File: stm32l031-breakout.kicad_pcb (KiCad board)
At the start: 2 copper layers, 12 parts, among them J1 Conn_01x16, J2 Conn_01x16, U1 STM32L031K6Tx

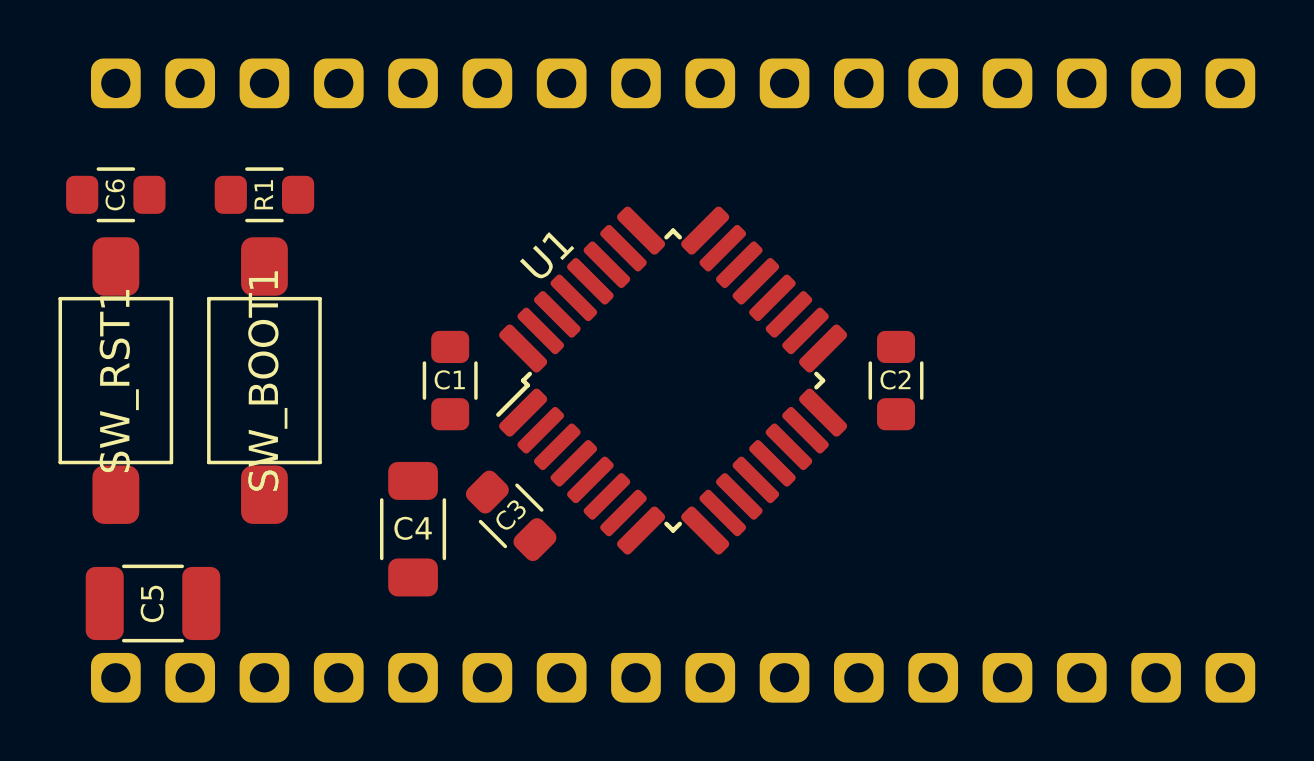
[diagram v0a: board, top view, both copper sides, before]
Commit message: Placement candidate
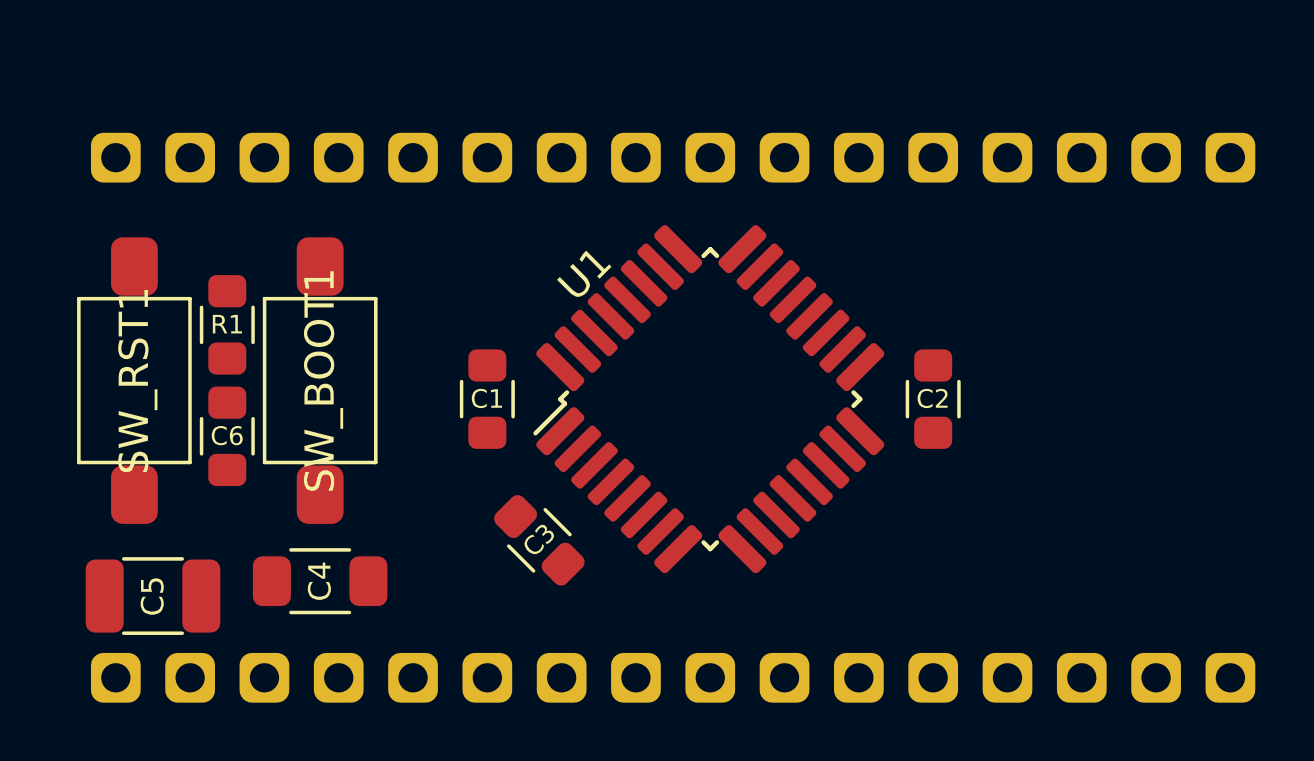
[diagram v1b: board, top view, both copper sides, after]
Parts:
- moved C6 9.09 mm to (143.5, 113.7), turned to 90 degrees
- moved R1 4.62 mm to (143.5, 109.9), turned to 270 degrees
- moved C4 3.64 mm to (146.7, 118.6), turned to 180 degrees
- moved J2 2.54 mm to (139.7, 104.1)
- moved SW_BOOT1 1.91 mm to (146.7, 111.8)
- moved C1 1.42 mm to (152.4, 112.4)
- moved U1 1.42 mm to (160.0, 112.4)
- moved C2 1.42 mm to (167.6, 112.4)
- moved C3 1.28 mm to (154.2, 117.2)
- moved SW_RST1 0.64 mm to (140.3, 111.8), turned to 270 degrees
- moved C5 0.25 mm to (141.0, 119.1)
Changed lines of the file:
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@@
   )
   (module local_footprints:0805_HS (layer F.Cu)
-    (at 151.13 111.76 90)
+    (at 152.4 112.395 90)
     (descr "Resistor SMD 0805, reflow soldering, Vishay (see dcrcw.pdf)")
     (tags "resistor 0805")
@@
   )
   (module local_footprints:0805_HS (layer F.Cu)
-    (at 166.37 111.76 270)
+    (at 167.64 112.395 270)
     (descr "Resistor SMD 0805, reflow soldering, Vishay (see dcrcw.pdf)")
     (tags "resistor 0805")
@@
   )
   (module local_footprints:0805_HS (layer F.Cu)
-    (at 153.213173 116.383173 135)
+    (at 154.178 117.221 135)
     (descr "Resistor SMD 0805, reflow soldering, Vishay (see dcrcw.pdf)")
     (tags "resistor 0805")
@@
   )
   (module local_footprints:1206_HS (layer F.Cu)
-    (at 149.86 116.84 90)
+    (at 146.685 118.618 180)
     (descr "Resistor SMD 1206, reflow soldering, Vishay (see dcrcw.pdf)")
     (tags "resistor 1206")
     (attr smd)
-    (fp_text reference C4 (at 0 0 180) (layer F.SilkS)
+    (fp_text reference C4 (at 0 0 270) (layer F.SilkS)
       (effects (font (size 0.762 0.762) (thickness 0.1016)))
     )
-    (fp_text value 1uF (at 0 1.95 90) (layer F.Fab) hide
+    (fp_text value 1uF (at 0 1.95 180) (layer F.Fab) hide
       (effects (font (size 1 1) (thickness 0.15)))
     )
@@
     (fp_line (start 1.6 0.8) (end -1.6 0.8) (layer F.Fab) (width 0.1))
     (fp_line (start -1.6 0.8) (end -1.6 -0.8) (layer F.Fab) (width 0.1))
-    (fp_text user %R (at 0 0 90) (layer F.Fab)
+    (fp_text user %R (at 0 0 180) (layer F.Fab)
       (effects (font (size 0.7 0.7) (thickness 0.105)))
     )
-    (pad 2 smd roundrect (at 1.65 0 90) (size 1.3 1.7) (layers F.Cu F.Paste F.Mask) (roundrect_rratio 0.25)
-      (net 2 GND))
-    (pad 1 smd roundrect (at -1.65 0 90) (size 1.3 1.7) (layers F.Cu F.Paste F.Mask) (roundrect_rratio 0.25)
+    (pad 2 smd roundrect (at 1.65 0 180) (size 1.3 1.7) (layers F.Cu F.Paste F.Mask) (roundrect_rratio 0.25)
+      (net 2 GND))
+    (pad 1 smd roundrect (at -1.65 0 180) (size 1.3 1.7) (layers F.Cu F.Paste F.Mask) (roundrect_rratio 0.25)
       (net 1 VDD))
     (model ${KISYS3DMOD}/Resistors_SMD.3dshapes/R_1206.wrl
@@
   )
   (module local_footprints:1210_HS (layer F.Cu)
-    (at 140.97 119.38)
+    (at 140.97 119.126)
     (descr "Generic SMD 1210")
     (tags "resistor 1206")
@@
   )
   (module local_footprints:0805_HS (layer F.Cu)
-    (at 139.7 105.41)
+    (at 143.51 113.665 90)
     (descr "Resistor SMD 0805, reflow soldering, Vishay (see dcrcw.pdf)")
     (tags "resistor 0805")
     (attr smd)
-    (fp_text reference C6 (at 0 0 90) (layer F.SilkS)
+    (fp_text reference C6 (at 0 0 180) (layer F.SilkS)
       (effects (font (size 0.635 0.635) (thickness 0.1016)))
     )
-    (fp_text value 0.1uF (at 0 1.75) (layer F.Fab) hide
-      (effects (font (size 1 1) (thickness 0.15)))
-    )
-    (fp_text user %R (at 0 0) (layer F.Fab)
+    (fp_text value 0.1uF (at 0 1.75 90) (layer F.Fab) hide
+      (effects (font (size 1 1) (thickness 0.15)))
+    )
+    (fp_text user %R (at 0 0 90) (layer F.Fab)
       (effects (font (size 0.5 0.5) (thickness 0.075)))
     )
@@
     (fp_line (start 1.55 0.9) (end 1.55 -0.9) (layer F.CrtYd) (width 0.05))
     (fp_line (start 1.55 0.9) (end -1.55 0.9) (layer F.CrtYd) (width 0.05))
-    (pad 1 smd roundrect (at -1.15 0) (size 1.1 1.3) (layers F.Cu F.Paste F.Mask) (roundrect_rratio 0.25)
+    (pad 1 smd roundrect (at -1.15 0 90) (size 1.1 1.3) (layers F.Cu F.Paste F.Mask) (roundrect_rratio 0.25)
       (net 3 "Net-(C6-Pad1)"))
-    (pad 2 smd roundrect (at 1.15 0) (size 1.1 1.3) (layers F.Cu F.Paste F.Mask) (roundrect_rratio 0.25)
+    (pad 2 smd roundrect (at 1.15 0 90) (size 1.1 1.3) (layers F.Cu F.Paste F.Mask) (roundrect_rratio 0.25)
       (net 2 GND))
     (model ${KISYS3DMOD}/Resistors_SMD.3dshapes/R_0805.wrl
@@
   )
   (module local_footprints:Pin_Header_Straight_1x16_Pitch2.54mm (layer F.Cu)
-    (at 139.7 101.6 90)
+    (at 139.7 104.14 90)
     (descr "Through hole straight pin header, 1x16, 2.54mm pitch, single row")
     (tags "Through hole pin header THT 1x16 2.54mm single row")
@@
   )
   (module local_footprints:0805_HS (layer F.Cu)
-    (at 144.78 105.41 180)
+    (at 143.51 109.855 270)
     (descr "Resistor SMD 0805, reflow soldering, Vishay (see dcrcw.pdf)")
     (tags "resistor 0805")
     (attr smd)
-    (fp_text reference R1 (at 0 0 270) (layer F.SilkS)
+    (fp_text reference R1 (at 0 0) (layer F.SilkS)
       (effects (font (size 0.635 0.635) (thickness 0.1016)))
     )
-    (fp_text value 10k (at 0 1.75 180) (layer F.Fab) hide
+    (fp_text value 10k (at 0 1.75 270) (layer F.Fab) hide
       (effects (font (size 1 1) (thickness 0.15)))
     )
@@
     (fp_line (start 1 0.62) (end -1 0.62) (layer F.Fab) (width 0.1))
     (fp_line (start -1 0.62) (end -1 -0.62) (layer F.Fab) (width 0.1))
-    (fp_text user %R (at 0 0 180) (layer F.Fab)
+    (fp_text user %R (at 0 0 270) (layer F.Fab)
       (effects (font (size 0.5 0.5) (thickness 0.075)))
     )
-    (pad 2 smd roundrect (at 1.15 0 180) (size 1.1 1.3) (layers F.Cu F.Paste F.Mask) (roundrect_rratio 0.25)
-      (net 2 GND))
-    (pad 1 smd roundrect (at -1.15 0 180) (size 1.1 1.3) (layers F.Cu F.Paste F.Mask) (roundrect_rratio 0.25)
+    (pad 2 smd roundrect (at 1.15 0 270) (size 1.1 1.3) (layers F.Cu F.Paste F.Mask) (roundrect_rratio 0.25)
+      (net 2 GND))
+    (pad 1 smd roundrect (at -1.15 0 270) (size 1.1 1.3) (layers F.Cu F.Paste F.Mask) (roundrect_rratio 0.25)
       (net 29 BOOT))
     (model ${KISYS3DMOD}/Resistors_SMD.3dshapes/R_0805.wrl
@@
   )
   (module local_footprints:SW_SPST_PUSH_6mm_3mm (layer F.Cu)
-    (at 144.78 111.76 270)
+    (at 146.685 111.76 270)
     (descr http://www.te.com/commerce/DocumentDelivery/DDEController?Action=srchrtrv&DocNm=1437566-3&DocType=Customer+Drawing&DocLang=English)
     (tags "SPST button tactile switch")
@@
   )
   (module local_footprints:SW_SPST_PUSH_6mm_3mm (layer F.Cu)
-    (at 139.7 111.76 90)
+    (at 140.335 111.76 270)
     (descr http://www.te.com/commerce/DocumentDelivery/DDEController?Action=srchrtrv&DocNm=1437566-3&DocType=Customer+Drawing&DocLang=English)
     (tags "SPST button tactile switch")
     (attr smd)
-    (fp_text reference SW_RST1 (at 0 0 90) (layer F.SilkS)
-      (effects (font (size 1 1) (thickness 0.15)))
-    )
-    (fp_text value SW_RST (at 0 3 90) (layer F.Fab)
+    (fp_text reference SW_RST1 (at 0 0 270) (layer F.SilkS)
+      (effects (font (size 1 1) (thickness 0.15)))
+    )
+    (fp_text value SW_RST (at 0 3 270) (layer F.Fab)
       (effects (font (size 1 1) (thickness 0.15)))
     )
@@
     (fp_line (start 1.75 -1) (end 1.75 1) (layer F.Fab) (width 0.1))
     (fp_line (start -1.75 -1) (end 1.75 -1) (layer F.Fab) (width 0.1))
-    (fp_text user %R (at 0 -2.6 90) (layer F.Fab)
-      (effects (font (size 1 1) (thickness 0.15)))
-    )
-    (pad 2 smd roundrect (at 3.9 0 90) (size 2 1.6) (layers F.Cu F.Paste F.Mask) (roundrect_rratio 0.25)
+    (fp_text user %R (at 0 -2.6 270) (layer F.Fab)
+      (effects (font (size 1 1) (thickness 0.15)))
+    )
+    (pad 2 smd roundrect (at 3.9 0 270) (size 2 1.6) (layers F.Cu F.Paste F.Mask) (roundrect_rratio 0.25)
       (net 3 "Net-(C6-Pad1)"))
-    (pad 1 smd roundrect (at -3.9 0 90) (size 2 1.6) (layers F.Cu F.Paste F.Mask) (roundrect_rratio 0.25)
+    (pad 1 smd roundrect (at -3.9 0 270) (size 2 1.6) (layers F.Cu F.Paste F.Mask) (roundrect_rratio 0.25)
       (net 2 GND))
     (model ${KISYS3DMOD}/Buttons_Switches_SMD.3dshapes/SW_SPST_FSMSM.wrl
@@
   )
   (module local_footprints:TQFP-32_7x7mm_Pitch0.8mm_HS_narrow_pads (layer F.Cu)
-    (at 158.75 111.76 45)
+    (at 160.02 112.395 45)
     (descr "32-Lead Plastic Thin Quad Flatpack (PT) - 7x7x1.0 mm Body, 2.00 mm [TQFP] (see Microchip Packaging Specification 00000049BS.pdf)")
     (tags "QFP 0.8")
